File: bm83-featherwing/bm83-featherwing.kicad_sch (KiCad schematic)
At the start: 1 part, among them U1 BM83SM1-00AA

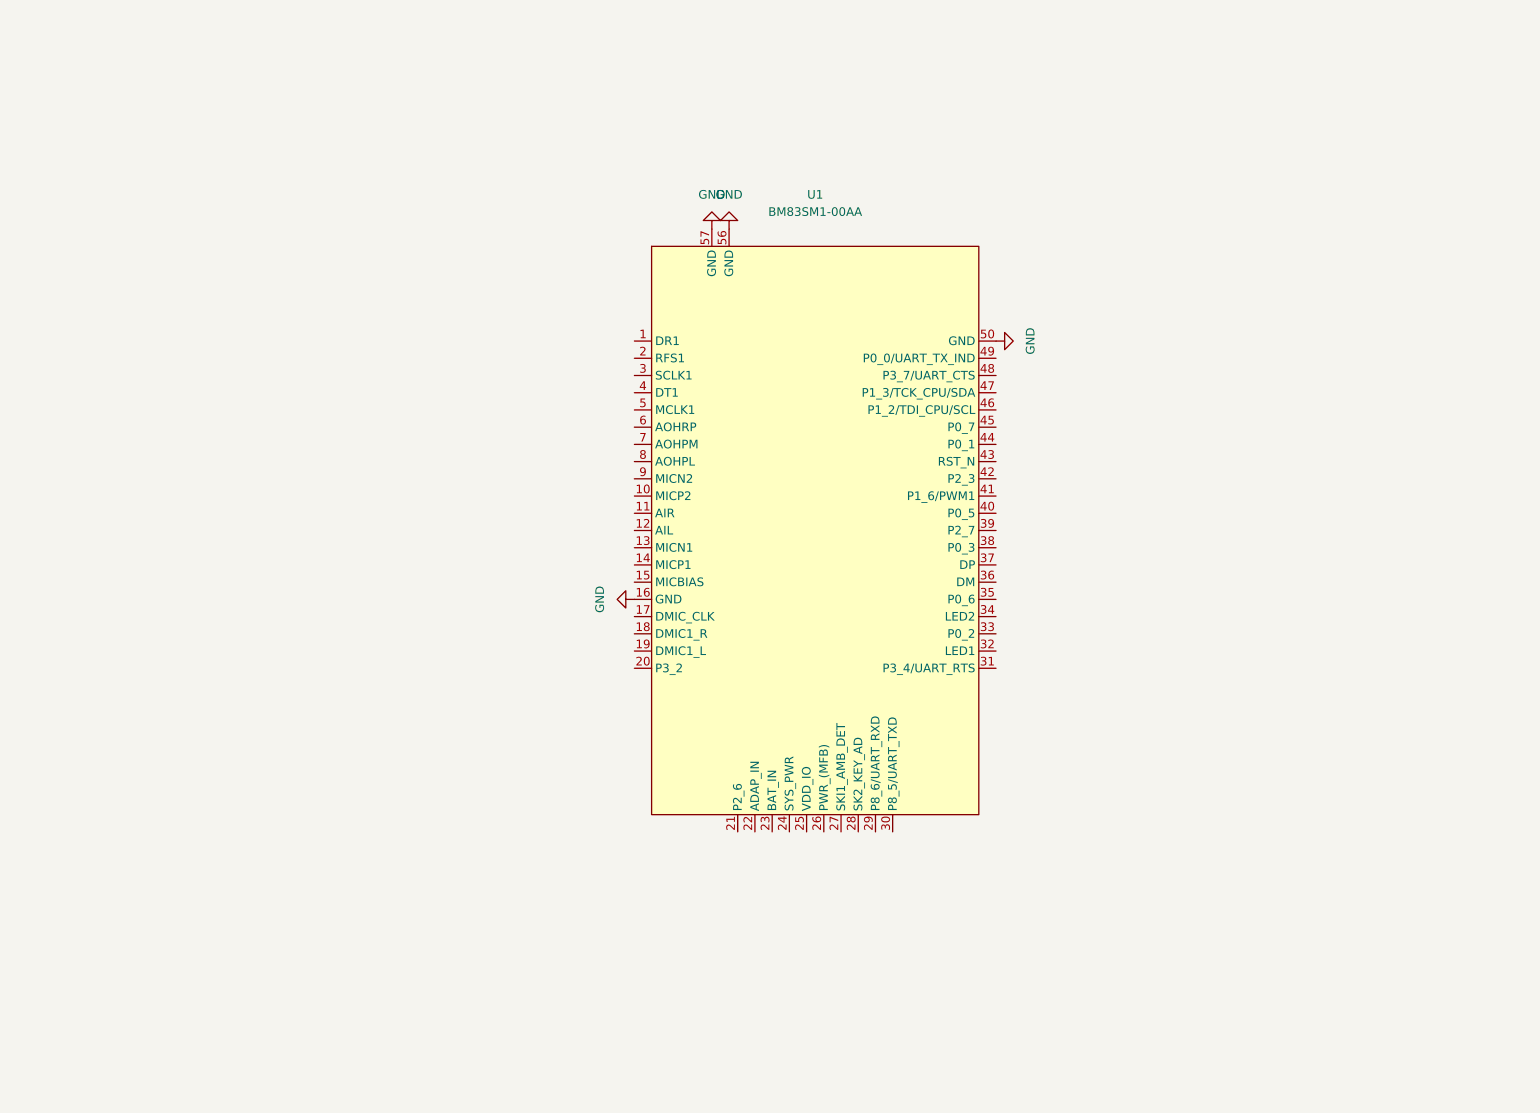
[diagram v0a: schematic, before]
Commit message: BM83 work
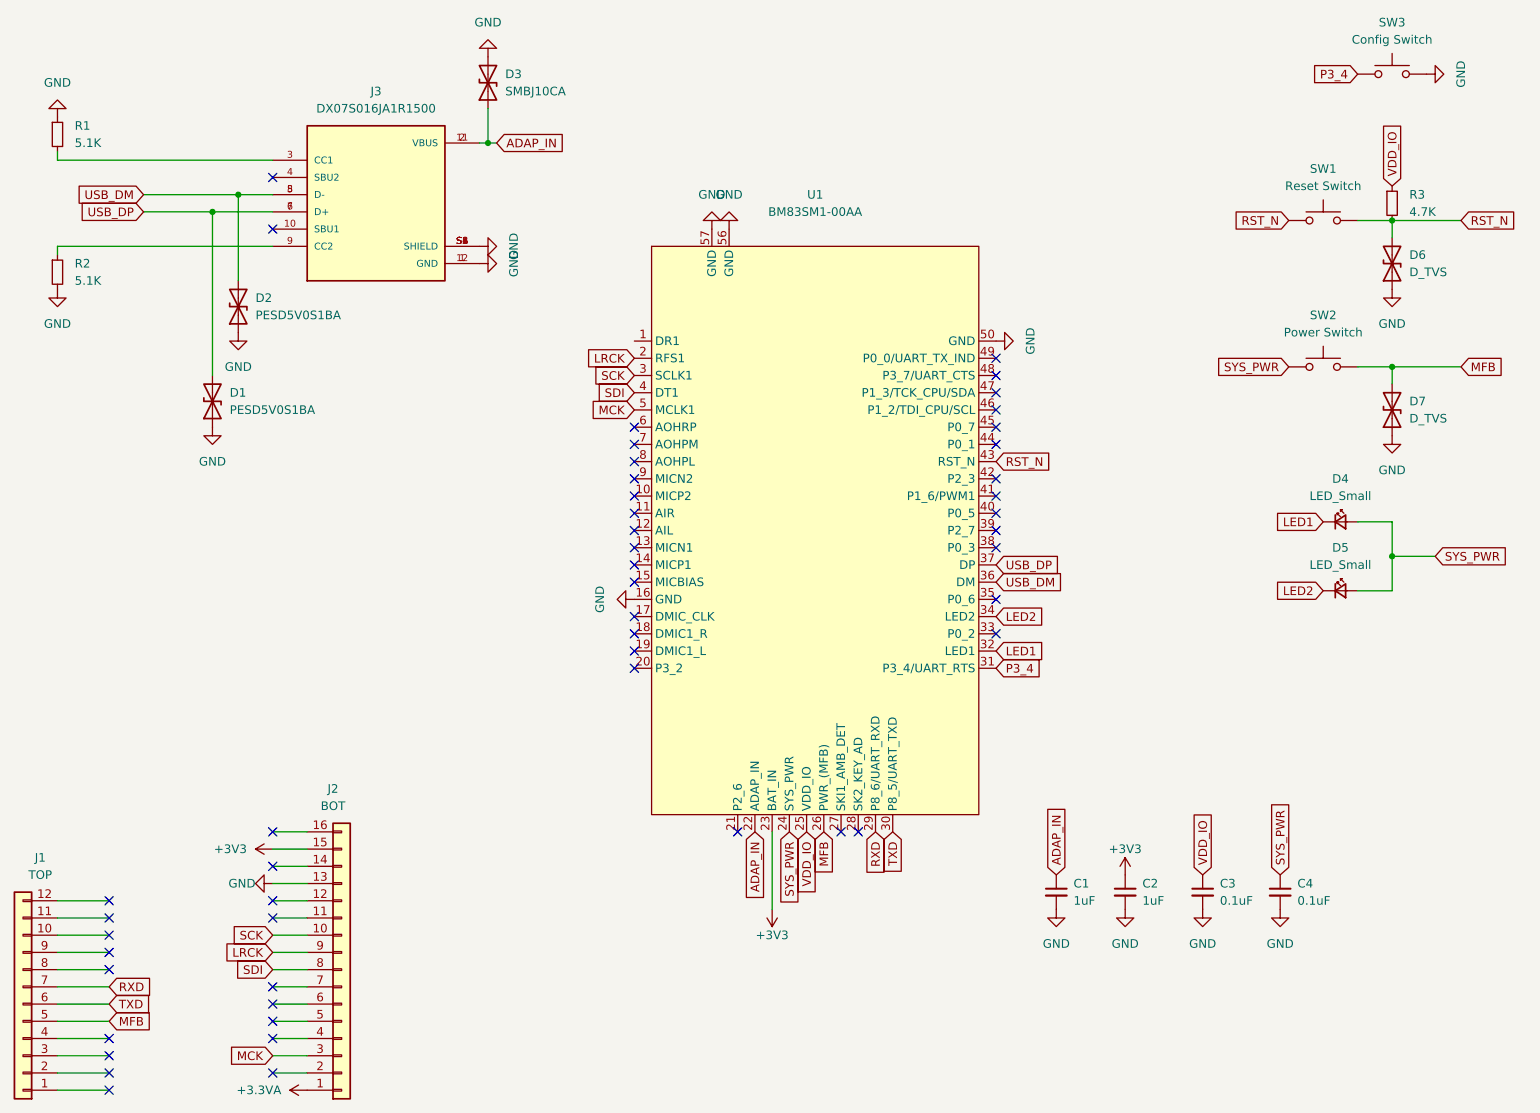
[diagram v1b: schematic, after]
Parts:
- added C1, C2: 1uF, Capacitor_SMD:C_0805_2012Metric_Pad1.18x1.45mm_HandSolder, symbol Device:C_Small
- added C3, C4: 0.1uF, Capacitor_SMD:C_0805_2012Metric_Pad1.18x1.45mm_HandSolder, symbol Device:C_Small
- added D1, D2: PESD5V0S1BA, Diode_SMD:D_SOD-323_HandSoldering, symbol Device:D_TVS
- added D3: SMBJ10CA, Diode_SMD:D_SMB_Handsoldering, symbol Device:D_TVS
- added D4, D5: LED_Small, LED_SMD:LED_0805_2012Metric_Pad1.15x1.40mm_HandSolder, symbol Device:LED_Small
- added D6, D7: D_TVS, Diode_SMD:D_SOD-323_HandSoldering, symbol Device:D_TVS
- added J1: TOP, Footprints:RoundPinHeader_1x12, symbol Connector_Generic:Conn_01x12
- added J2: BOT, Footprints:RoundPinHeader_1x16, symbol Connector_Generic:Conn_01x16
- added J3: DX07S016JA1R1500, Footprints:JAE_DX07S016JA1R1500, symbol DX07S016JA1R1500:DX07S016JA1R1500
- added R1, R2: 5.1K, Resistor_SMD:R_0805_2012Metric_Pad1.20x1.40mm_HandSolder, symbol Device:R_Small
- added R3: 4.7K, Resistor_SMD:R_0805_2012Metric_Pad1.20x1.40mm_HandSolder, symbol Device:R_Small
- added SW1: Reset Switch, Footprints:PTS636SK25SMTRLFS, symbol Switch:SW_Push
- added SW2: Power Switch, Footprints:PTS636SK25SMTRLFS, symbol Switch:SW_Push
- added SW3: Config Switch, Footprints:PTS636SK25SMTRLFS, symbol Switch:SW_Push
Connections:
- net GND: now also C1.2, C2.2, C3.2, C4.2, D1.1 (A1), D2.1 (A1), D3.2 (A2), D6.1 (A1), D7.1 (A1), J2.13 (Pin_13), J3.1 (GND), J3.12 (GND), J3.S1 (SHIELD), J3.S2 (SHIELD), J3.S3 (SHIELD), J3.S4 (SHIELD), J3.S5 (SHIELD), J3.S6 (SHIELD), R1.1, R2.2, SW3.2
- net LRCK: now reaches U1.2 (RFS1)
- net LRCK: now also J2.9 (Pin_9)
- net ADAP_IN: now reaches U1.22 (ADAP_IN)
- net ADAP_IN: now also C1.1, D3.1 (A1), J3.11 (VBUS), J3.2 (VBUS)
- net +3V3: now reaches U1.23 (BAT_IN)
- net +3V3: now also C2.1, J2.15 (Pin_15)
- net SYS_PWR: now reaches U1.24 (SYS_PWR)
- net SYS_PWR: now also C4.1, D4.2 (A), D5.2 (A), SW2.1
- net VDD_IO: now reaches U1.25 (VDD_IO)
- net VDD_IO: now also C3.1, R3.1
- net MFB: now reaches U1.26 (PWR_(MFB))
- net MFB: now also D7.2 (A2), J1.5 (Pin_5), SW2.2
- net RXD: now reaches U1.29 (P8_6/UART_RXD)
- net RXD: now also J1.7 (Pin_7)
- net SCK: now reaches U1.3 (SCLK1)
- net SCK: now also J2.10 (Pin_10)
- net TXD: now reaches U1.30 (P8_5/UART_TXD)
- net TXD: now also J1.6 (Pin_6)
- net P3_4: now reaches U1.31 (P3_4/UART_RTS)
- net P3_4: now also SW3.1
- net LED1: now reaches U1.32 (LED1)
- net LED1: now also D4.1 (K)
- net LED2: now reaches U1.34 (LED2)
- net LED2: now also D5.1 (K)
- net USB_DM: now reaches U1.36 (DM)
- net USB_DM: now also D2.2 (A2), J3.5 (D-), J3.8 (D-)
- net USB_DP: now reaches U1.37 (DP)
- net USB_DP: now also D1.2 (A2), J3.6 (D+), J3.7 (D+)
- net SDI: now reaches U1.4 (DT1)
- net SDI: now also J2.8 (Pin_8)
- net RST_N: now reaches U1.43 (RST_N)
- net RST_N: now also D6.2 (A2), R3.2, SW1.1, SW1.2
- net MCK: now reaches U1.5 (MCLK1)
- net MCK: now also J2.3 (Pin_3)
- new net: J3.3 (CC1), R1.2
- new net: J3.9 (CC2), R2.1
- new net +3.3VA: J2.1 (Pin_1)
- no-connect marks 0 -> 50
